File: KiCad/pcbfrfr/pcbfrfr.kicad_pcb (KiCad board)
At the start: 2 copper layers, 68 x 91.5 mm, 40 parts, among them J1 Barrel_Jack_Switch, J10 Conn_01x05_Pin, J11 Conn_01x05_Pin, J12 Conn_01x04_Pin, J13 Conn_01x04_Pin, J14 Conn_01x04_Pin, J15 Conn_01x04_Pin, J16 Conn_01x05_Pin, J17 Conn_01x05_Pin, J18 Conn_01x05_Pin, J19 Conn_01x05_Pin, J2 Conn_01x02_Pin, J20 Conn_01x05_Pin, J21 Conn_01x02_Pin, J3 Conn_01x19_Socket, J4 Conn_01x19_Socket, J5 Conn_01x19_Socket, J6 Conn_01x05_Pin, J7 Conn_01x19_Socket, J8 Conn_01x04_Pin, J9 Conn_01x03_Pin, U1 AP63203WU, U2 AP63205WU

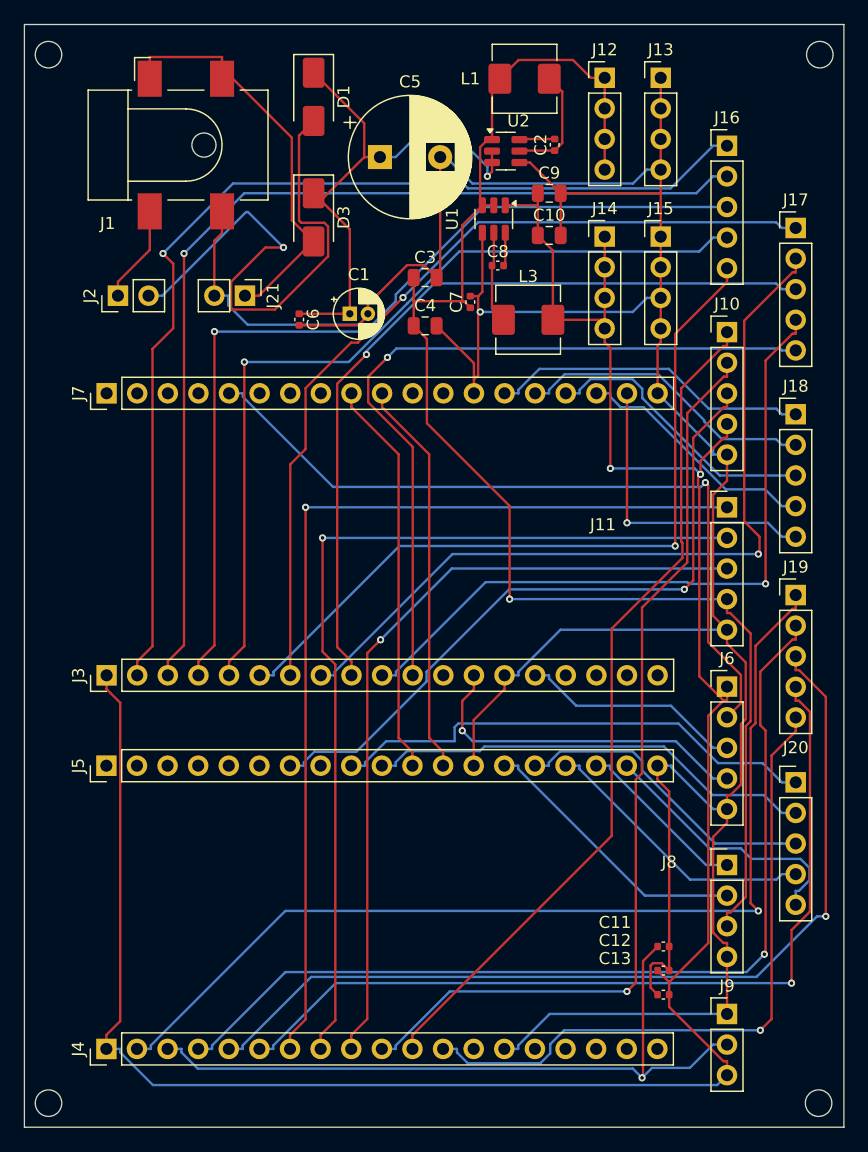
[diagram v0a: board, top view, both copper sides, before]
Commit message: updatedpcb
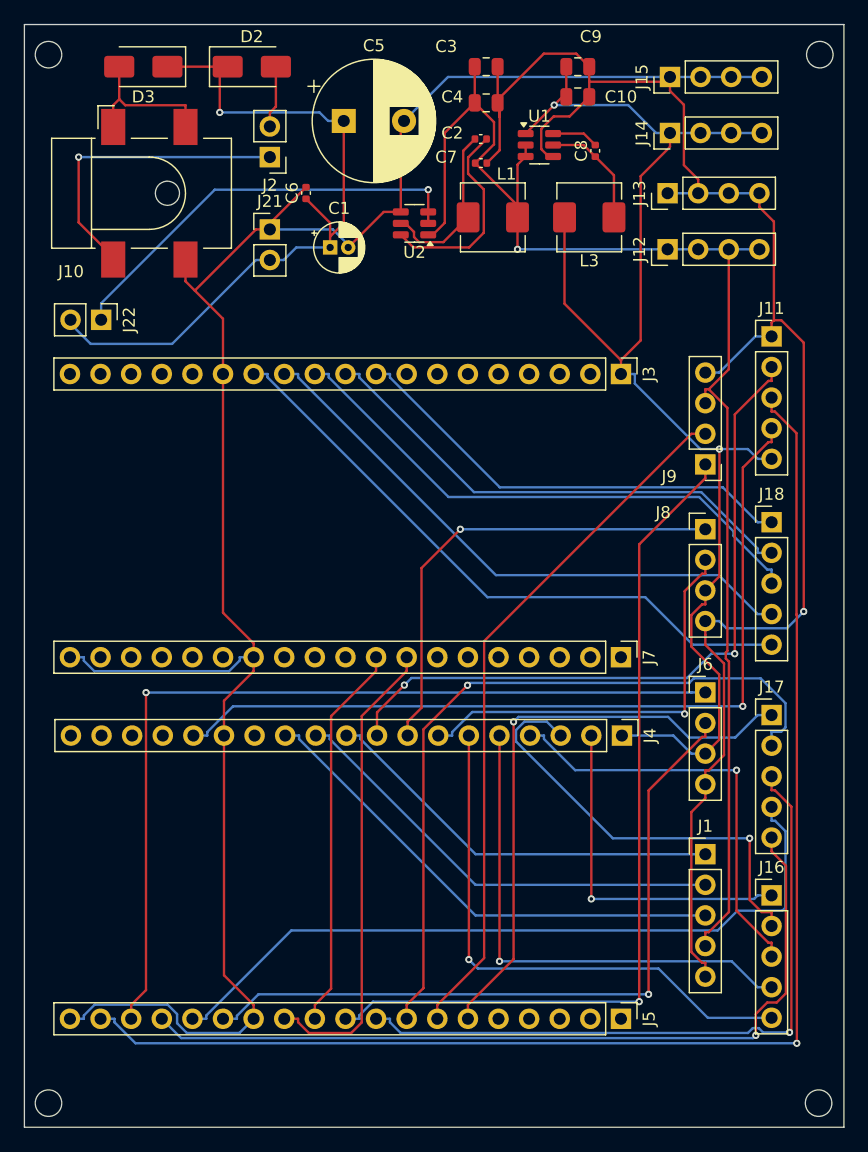
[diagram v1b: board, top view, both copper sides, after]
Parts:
- removed C11: 0.001 uF, Capacitor_SMD:C_0402_1005Metric
- removed C12, C13: 0.1 uF, Capacitor_SMD:C_0402_1005Metric
- removed D1: SS24, Diode_SMD:D_SMA
- removed J19, J20: Conn_01x05_Pin, Connector_PinHeader_2.54mm:PinHeader_1x05_P2.54mm_Vertical
- added D2: US2AA, Diode_SMD:D_SMA, F.Cu at (137.9, 35.5)
- added J22: estop, Connector_PinHeader_2.54mm:PinHeader_1x02_P2.54mm_Vertical, F.Cu at (125.4, 56.5)
- J1: value Barrel_Jack_Switch -> Conn_01x05_Pin; footprint Connector_BarrelJack:BarrelJack_CLIFF_FC681465S_SMT_Horizontal -> Connector_PinHeader_2.54mm:PinHeader_1x05_P2.54mm_Vertical
- J10: value Conn_01x05_Pin -> Barrel_Jack_Switch; footprint Connector_PinHeader_2.54mm:PinHeader_1x05_P2.54mm_Vertical -> Connector_BarrelJack:BarrelJack_CLIFF_FC681465S_SMT_Horizontal
- J2: value Conn_01x02_Pin -> battery
- J21: value Conn_01x02_Pin -> mtr
- J6: value Conn_01x05_Pin -> Conn_01x04_Pin; footprint Connector_PinHeader_2.54mm:PinHeader_1x05_P2.54mm_Vertical -> Connector_PinHeader_2.54mm:PinHeader_1x04_P2.54mm_Vertical
- J9: value Conn_01x03_Pin -> Conn_01x04_Pin; footprint Connector_PinHeader_2.54mm:PinHeader_1x03_P2.54mm_Vertical -> Connector_PinHeader_2.54mm:PinHeader_1x04_P2.54mm_Vertical
- moved J1 72.9 mm to (175.5, 100.8)
- moved J16 62.3 mm to (181.0, 104.3)
- moved J4 50.1 mm to (168.6, 91.0), turned to -90 degrees
- moved J3 49.5 mm to (168.5, 61.0), turned to -90 degrees
- moved J10 49.3 mm to (129.4, 46.0)
- moved J7 48.0 mm to (168.5, 84.5), turned to -90 degrees
- moved J5 47.6 mm to (168.5, 114.5), turned to -90 degrees
- moved J9 45.6 mm to (175.5, 68.5), turned to 180 degrees
- moved J17 40.5 mm to (181.0, 89.3)
- moved J8 27.9 mm to (175.5, 73.9)
- moved C4 19.2 mm to (157.3, 38.5)
- moved D3 18.9 mm to (128.9, 35.5), turned to 180 degrees
- moved C3 18.2 mm to (157.3, 35.5)
- moved J2 17.1 mm to (139.4, 43.0), turned to 180 degrees
- moved J12 15.2 mm to (172.4, 50.6), turned to 90 degrees
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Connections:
- C1 pad 1: Net-(D1-K) -> Net-(D2-K)
- C10 pad 1: 3.3V -> Net-(J11-Pin_5)
- C3 pad 1: Net-(J11-Pin_4) -> Net-(J1-Pin_4)
- C4 pad 1: Net-(J11-Pin_4) -> Net-(J1-Pin_4)
- C5 pad 1: Net-(D1-K) -> Net-(D2-K)
- C6 pad 1: Net-(D1-K) -> Net-(D2-K)
- C7 pad 1: Net-(J11-Pin_4) -> Net-(J1-Pin_4)
- C9 pad 1: 3.3V -> Net-(J11-Pin_5)
- D3 pad 1: Net-(D1-K) -> Net-(D2-K)
- J1 pad 1: Net-(D3-A) -> Net-(J1-Pin_1)
- J1 pad 2: GND -> Net-(J1-Pin_2)
- J1 pad 3: Net-(J2-Pin_1) -> Net-(J1-Pin_3)
- J10 pad 1: Net-(J10-Pin_1) -> Net-(D3-A)
- J10 pad 2: Net-(J10-Pin_2) -> GND
- J10 pad 3: Net-(J10-Pin_3) -> Net-(J2-Pin_1)
- J11 pad 1: Net-(J11-Pin_1) -> GND
- J11 pad 5: GND -> Net-(J11-Pin_5)
- J12 pad 1: Net-(J11-Pin_4) -> Net-(J1-Pin_4)
- J12 pad 2: Net-(J11-Pin_4) -> Net-(J1-Pin_4)
- J12 pad 3: Net-(J11-Pin_4) -> Net-(J1-Pin_4)
- J12 pad 4: Net-(J11-Pin_4) -> Net-(J1-Pin_4)
- J14 pad 1: 3.3V -> Net-(J11-Pin_5)
- J14 pad 2: 3.3V -> Net-(J11-Pin_5)
- J14 pad 3: 3.3V -> Net-(J11-Pin_5)
- J14 pad 4: 3.3V -> Net-(J11-Pin_5)
- J17 pad 4: Net-(J17-Pin_4) -> /screen
- J21 pad 1: Net-(D3-A) -> GND
- J21 pad 2: GND -> Net-(D2-K)
- J3 pad 1: 3.3V -> Net-(J11-Pin_5)
- J3 pad 10: Net-(J17-Pin_4) -> Net-(J18-Pin_2)
- J3 pad 11: Net-(J17-Pin_5) -> Net-(J18-Pin_3)
- J3 pad 12: unconnected-(J3-Pin_12-Pad12) -> Net-(J18-Pin_4)
- J3 pad 13: Net-(J3-Pin_13) -> Net-(J18-Pin_5)
- J3 pad 15: Net-(J3-Pin_15) -> unconnected-(J3-Pin_15-Pad15)
- J3 pad 2: Net-(J16-Pin_1) -> unconnected-(J3-Pin_2-Pad2)
- J3 pad 3: Net-(J16-Pin_2) -> unconnected-(J3-Pin_3-Pad3)
- J3 pad 4: Net-(J16-Pin_3) -> unconnected-(J3-Pin_4-Pad4)
- J3 pad 5: Net-(J16-Pin_4) -> unconnected-(J3-Pin_5-Pad5)
- J3 pad 6: Net-(J16-Pin_5) -> unconnected-(J3-Pin_6-Pad6)
- J3 pad 7: Net-(J17-Pin_1) -> unconnected-(J3-Pin_7-Pad7)
- J3 pad 8: Net-(J17-Pin_2) -> unconnected-(J3-Pin_8-Pad8)
- J3 pad 9: Net-(J17-Pin_3) -> Net-(J18-Pin_1)
- J4 pad 1: 3.3V -> Net-(J11-Pin_5)
- J4 pad 10: Net-(J10-Pin_2) -> Net-(J1-Pin_1)
- J4 pad 11: Net-(J10-Pin_1) -> Net-(J1-Pin_2)
- J4 pad 12: Net-(J19-Pin_5) -> Net-(J1-Pin_3)
- J4 pad 15: unconnected-(J4-Pin_15-Pad15) -> Net-(J11-Pin_4)
- J4 pad 2: Net-(J19-Pin_1) -> Net-(J16-Pin_1)
- J4 pad 3: Net-(J4-Pin_3) -> Net-(J16-Pin_2)
- J4 pad 4: Net-(J19-Pin_2) -> Net-(J16-Pin_3)
- J4 pad 5: Net-(J19-Pin_3) -> Net-(J16-Pin_4)
- J4 pad 6: Net-(J19-Pin_4) -> Net-(J16-Pin_5)
- J4 pad 7: Net-(J11-Pin_1) -> Net-(J4-Pin_7)
- J4 pad 8: Net-(J11-Pin_2) -> Net-(J4-Pin_8)
- J4 pad 9: Net-(J11-Pin_3) -> Net-(J11-Pin_2)
- J5 pad 10: Net-(J20-Pin_2) -> Net-(J5-Pin_10)
- J5 pad 15: Net-(J20-Pin_3) -> /screen
- J5 pad 16: Net-(J20-Pin_4) -> Net-(J17-Pin_5)
- J5 pad 18: Net-(J20-Pin_5) -> Net-(J11-Pin_3)
- J5 pad 6: unconnected-(J5-Pin_6-Pad6) -> Net-(J17-Pin_1)
- J5 pad 7: Net-(J10-Pin_3) -> Net-(J5-Pin_7)
- J5 pad 8: unconnected-(J5-Pin_8-Pad8) -> Net-(J17-Pin_2)
- J5 pad 9: Net-(J20-Pin_1) -> Net-(J17-Pin_3)
- J6 pad 1: 3.3V -> Net-(J5-Pin_17)
- J6 pad 2: Net-(J6-Pin_2) -> Net-(J5-Pin_14)
- J6 pad 3: Net-(J3-Pin_15) -> Net-(J11-Pin_5)
- J6 pad 4: Net-(J3-Pin_13) -> GND
- J7 pad 10: Net-(J5-Pin_12) -> unconnected-(J7-Pin_10-Pad10)
- J7 pad 14: Net-(J18-Pin_1) -> unconnected-(J7-Pin_14-Pad14)
- J7 pad 15: Net-(J18-Pin_2) -> unconnected-(J7-Pin_15-Pad15)
- J7 pad 16: Net-(J18-Pin_3) -> unconnected-(J7-Pin_16-Pad16)
- J7 pad 17: Net-(J18-Pin_4) -> unconnected-(J7-Pin_17-Pad17)
- J7 pad 18: Net-(J18-Pin_5) -> unconnected-(J7-Pin_18-Pad18)
- J7 pad 5: Net-(J6-Pin_2) -> unconnected-(J7-Pin_5-Pad5)
- J7 pad 8: unconnected-(J7-Pin_8-Pad8) -> Net-(J5-Pin_12)
- J8 pad 1: Net-(J5-Pin_17) -> Net-(J4-Pin_8)
- J8 pad 2: Net-(J5-Pin_14) -> Net-(J4-Pin_7)
- J8 pad 3: Net-(J11-Pin_4) -> Net-(J11-Pin_5)
- J9 pad 1: GND -> Net-(J5-Pin_10)
- J9 pad 2: Net-(J4-Pin_3) -> Net-(J5-Pin_7)
- J9 pad 3: 3.3V -> Net-(J1-Pin_4)
- L1 pad 2: Net-(J11-Pin_4) -> Net-(J1-Pin_4)
- L3 pad 2: 3.3V -> Net-(J11-Pin_5)
- U1 pad 1: 3.3V -> Net-(J11-Pin_5)
- U1 pad 2: Net-(J11-Pin_4) -> Net-(J1-Pin_4)
- U1 pad 3: Net-(J11-Pin_4) -> Net-(J1-Pin_4)
- U2 pad 1: Net-(J11-Pin_4) -> Net-(J1-Pin_4)
- U2 pad 2: Net-(D1-K) -> Net-(J22-Pin_1)
- U2 pad 3: Net-(D1-K) -> Net-(J22-Pin_1)
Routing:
- net 3.3V: track 193.2 -> 0.00 mm, vias 2 -> 0
- net Net-(J1-Pin_4): track 0.00 -> 118.8 mm, vias 0 -> 1
- net Net-(J11-Pin_5): track 0.00 -> 112.0 mm, vias 0 -> 2
- net Net-(J19-Pin_1): track 84.7 -> 0.00 mm, vias 1 -> 0
- net Net-(J11-Pin_1): track 80.4 -> 0.00 mm, vias 1 -> 0
- net Net-(J19-Pin_2): track 79.3 -> 0.00 mm, vias 1 -> 0
- net Net-(J10-Pin_2): track 78.2 -> 0.00 mm, vias 1 -> 0
- net Net-(J19-Pin_3): track 77.0 -> 0.00 mm, vias 1 -> 0
- net Net-(J19-Pin_4): track 72.4 -> 0.00 mm, vias 1 -> 0
- net Net-(J5-Pin_10): track 0.00 -> 72.0 mm, vias 0 -> 1
- net Net-(J10-Pin_1): track 70.5 -> 0.00 mm
- net Net-(J6-Pin_2): track 64.2 -> 0.00 mm, vias 1 -> 0
- net /screen: track 0.00 -> 62.2 mm
- net Net-(D2-K): track 0.00 -> 60.5 mm, vias 0 -> 1
- net Net-(J4-Pin_3): track 60.2 -> 0.00 mm, vias 1 -> 0
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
